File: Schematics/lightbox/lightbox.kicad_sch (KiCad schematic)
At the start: 40 parts, among them J1 Conn_01x07_Female, J2 Screw_Terminal_01x03, J3 Conn_01x12_Female, J4 Conn_01x12_Female, Q1 IRF740, SW1 SW_SP3T, SW3 SW_Push_Reset, SW4 SW_Push_+, U1 ATtiny85-20P, U2 LM317_TO-220, U3 74AHCT595, U4 74HC595, U5 D148K, U6 D148K, U7 D148K, U8 D148K

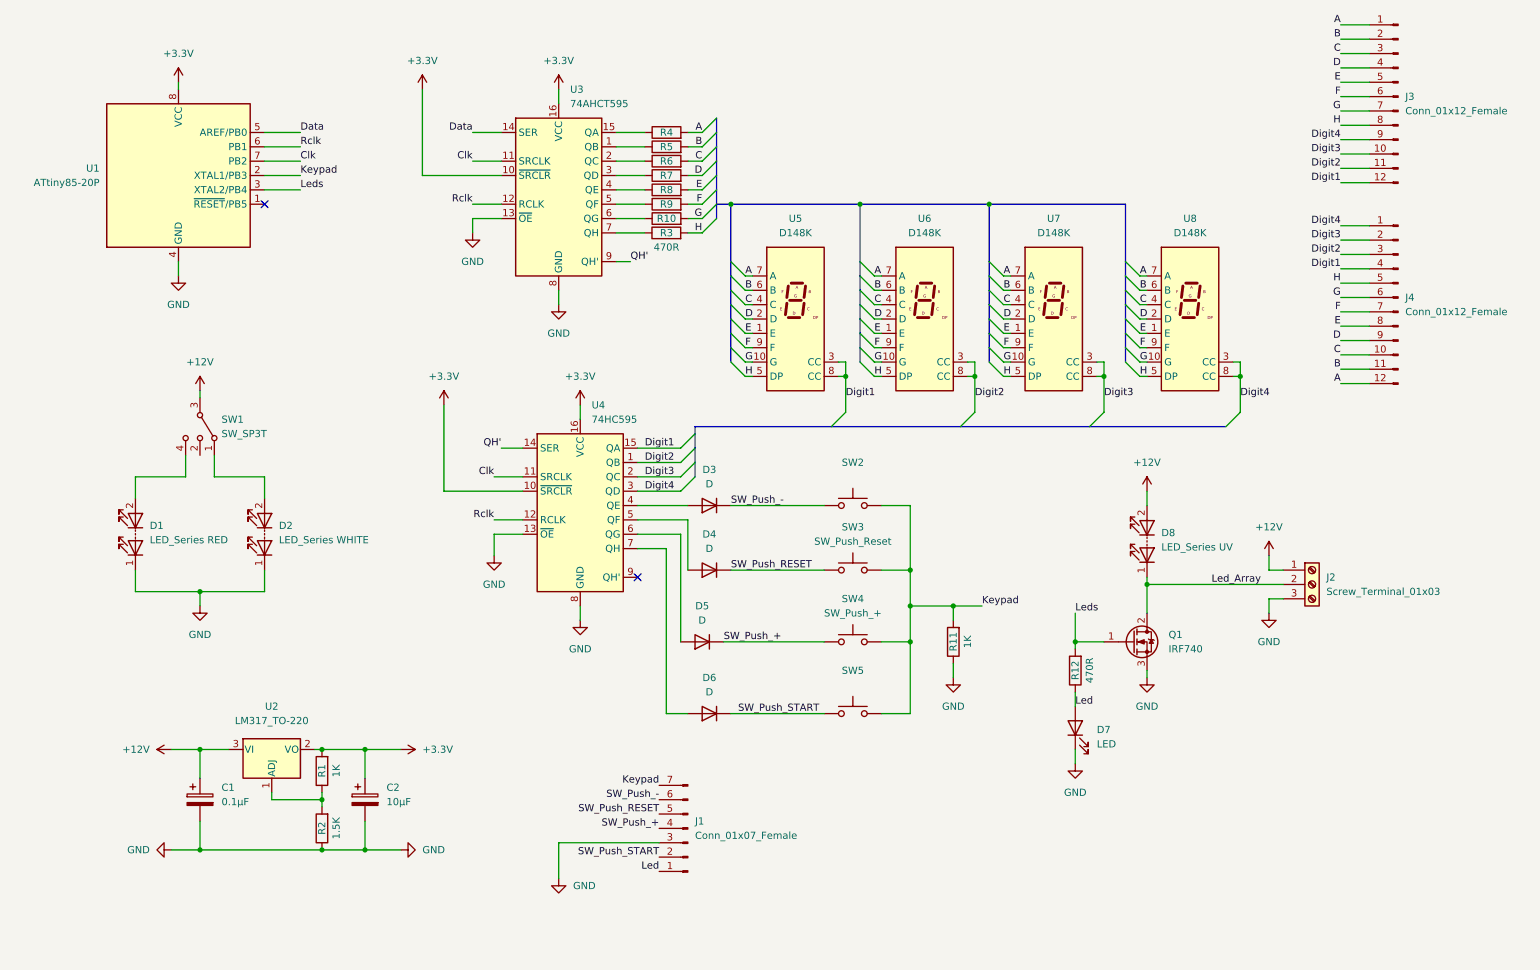
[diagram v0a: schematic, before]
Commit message: Update Schematic and PCB layout
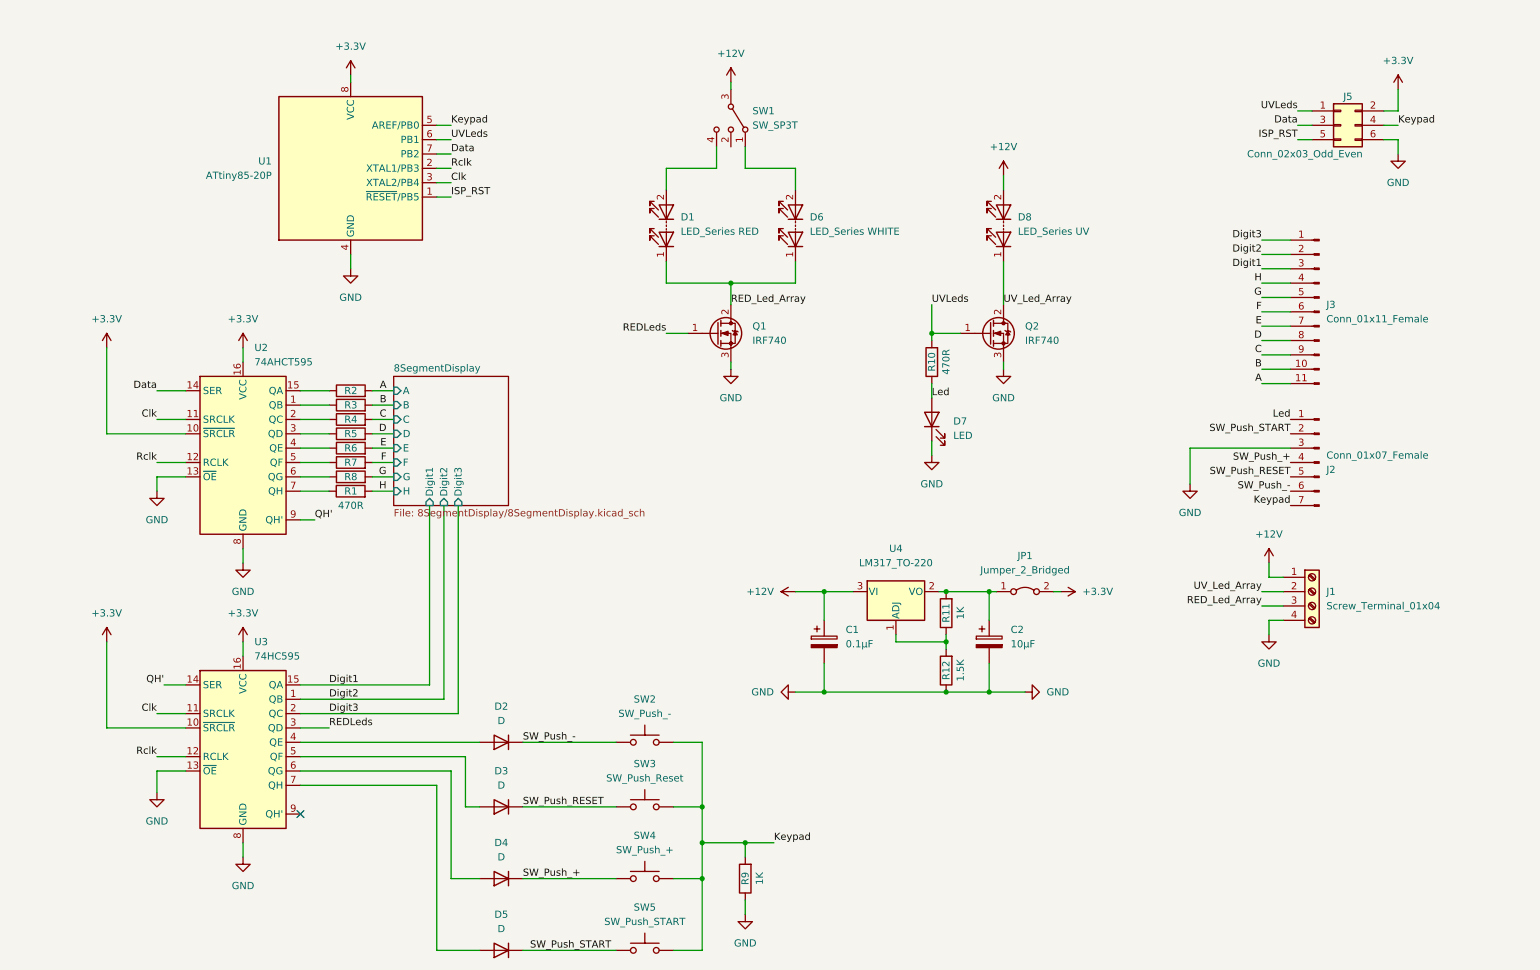
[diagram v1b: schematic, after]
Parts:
- removed J3, J4: Conn_01x12_Female, Connector_PinHeader_1.27mm:PinHeader_1x12_P1.27mm_Horizontal, symbol Connector:Conn_01x12_Male
- removed U5, U6, U7, U8: D148K, Display_7Segment:D1X8K, symbol Display_Character:D148K
- added J3: Conn_01x11_Female, Connector_PinHeader_1.27mm:PinHeader_1x12_P1.27mm_Horizontal, symbol Connector:Conn_01x11_Male
- added J5: Conn_02x03_Odd_Even, Connector_PinHeader_1.27mm:PinHeader_2x03_P1.27mm_Vertical, symbol Connector_Generic:Conn_02x03_Odd_Even
- added JP1: Jumper_2_Bridged, Connector_PinHeader_1.27mm:PinHeader_1x02_P1.27mm_Vertical, symbol Jumper:Jumper_2_Bridged
- added Q1: IRF740, Package_TO_SOT_THT:TO-220-3_Vertical, symbol Transistor_FET:IRF740
- J1: renamed from J2; value Screw_Terminal_01x03 -> Screw_Terminal_01x04; footprint TerminalBlock:TerminalBlock_Altech_AK300-3_P5.00mm -> TerminalBlock:TerminalBlock_Altech_AK300-4_P5.00mm; symbol Connector:Screw_Terminal_01x03 -> Connector:Screw_Terminal_01x04
- SW2: value (none) -> SW_Push_-
- SW5: value (none) -> SW_Push_START
- renumbered D3 to D2, D4 to D3, D5 to D4, D6 to D5, D2 to D6, J1 to J2, Q1 to Q2, R3 to R1, R12 to R10, R1 to R11, R2 to R12, R4 to R2, R5 to R3, R6 to R4, R7 to R5, R8 to R6, R9 to R7, R10 to R8, R11 to R9, U3 to U2, U4 to U3, U2 to U4
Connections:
- net +3V3: now also J5.2 (Pin_2), JP1.2 (B); no longer C2.1, R11.2, U4.2 (VO)
- net A: now also J3.11 (Pin_11)
- net B: now also J3.10 (Pin_10)
- net C: now also J3.9 (Pin_9)
- net Clk: now also U1.3 (XTAL2/PB4); no longer U1.7 (PB2)
- net D: now also J3.8 (Pin_8)
- net Data: now also U1.7 (PB2), J5.3 (Pin_3); no longer U1.5 (AREF/PB0)
- net Digit1: now also J3.3 (Pin_3)
- net Digit2: now also J3.2 (Pin_2)
- net Digit3: now also J3.1 (Pin_1)
- net E: now also J3.7 (Pin_7)
- net F: now also J3.6 (Pin_6)
- net G: now also J3.5 (Pin_5)
- net GND: now also J1.4 (Pin_4), J5.6 (Pin_6), Q1.3 (S); no longer D1.1 (K), D6.1 (K), J1.3 (Pin_3)
- net H: now also J3.4 (Pin_4)
- net Keypad: now also U1.5 (AREF/PB0), J5.4 (Pin_4); no longer U1.2 (XTAL1/PB3)
- net Rclk: now also U1.2 (XTAL1/PB3); no longer U1.6 (PB1)
- net ISP_RST: now reaches U1.1 (~{RESET}/PB5)
- net ISP_RST: now also J5.5 (Pin_5)
- net Digit4 renamed REDLeds
- net REDLeds: now also Q1.1 (G)
- net Led_Array renamed UV_Led_Array
- net Leds renamed UVLeds
- net UVLeds: now also U1.6 (PB1), J5.1 (Pin_1); no longer U1.3 (XTAL2/PB4)
- new net: C2.1, JP1.1 (A), R11.2, U4.2 (VO)
- new net RED_Led_Array: D1.1 (K), D6.1 (K), J1.3 (Pin_3), Q1.2 (D)
- no-connect marks 2 -> 1
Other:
- added sheet 8SegmentDisplay (8SegmentDisplay/8SegmentDisplay.kicad_sch)
- moved on the sheet: C1, C2, D1, D2, D3, D4, D5, D6, D7, D8, J2, Q2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
